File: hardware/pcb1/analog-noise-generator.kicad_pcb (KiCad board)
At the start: 4 copper layers, 12.7 x 53 mm, 79 parts, among them J1 USB_C_Receptacle_USB2.0, J2 Conn_01x03_Pin, J5 Conn_01x04_Pin, J6 Conn_01x04_Pin, J7 Conn_01x02_Pin, J9 Conn_02x04_Odd_Even, U1 STM32F072CBTx, U2 USBLC6-2SC6, U3 LR8321A-T33, U4 LIS2DH12, U5 LM324

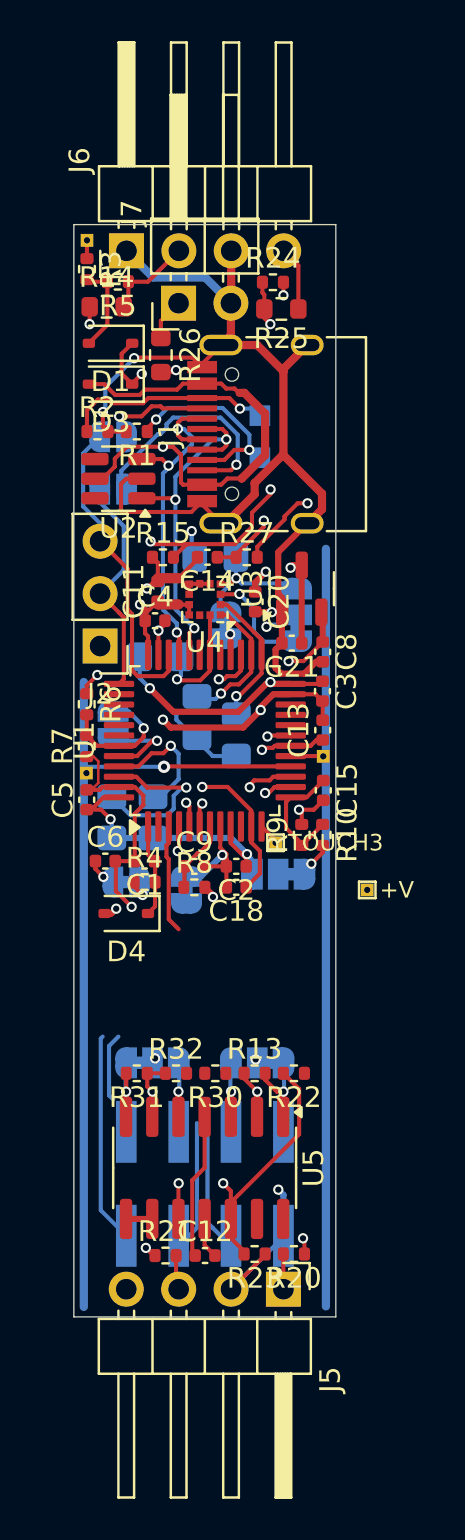
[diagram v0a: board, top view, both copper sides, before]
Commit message: finish routing
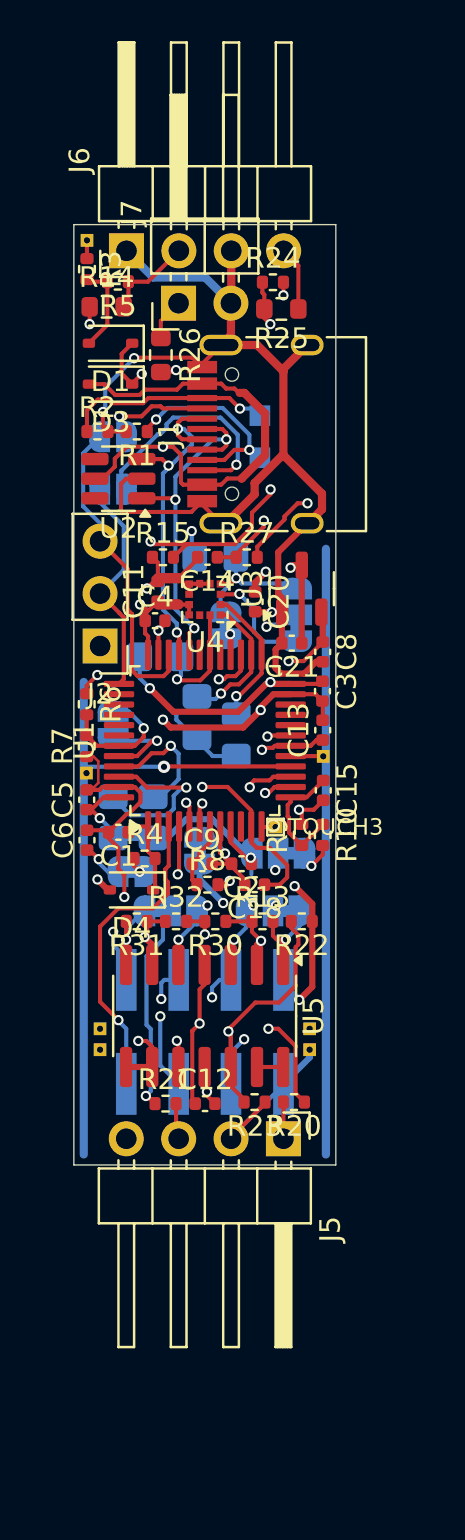
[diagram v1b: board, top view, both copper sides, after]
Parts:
- added TP10: AGND, analog-noise-generator:TestPoint_THTPad_small, B.Cu at (106.7, 96.5)
- added TP11: AVCC, analog-noise-generator:TestPoint_THTPad_small, B.Cu at (106.7, 95.5)
- added TP9: GND, analog-noise-generator:TestPoint_THTPad_small, B.Cu at (116.8, 96.5)
- TP4: moved to B.Cu
- moved JP6 7.42 mm to (110.1, 89.8)
- moved JP4 7.41 mm to (115.1, 89.8)
- moved R13 7.38 mm to (114.6, 90.3)
- moved R22 7.38 mm to (116.5, 90.3)
- moved C12 7.37 mm to (111.8, 99.1)
- moved J9 7.37 mm to (111.8, 95.7)
- moved R20 7.37 mm to (116.1, 99.1)
- moved R21 7.37 mm to (109.9, 99.1)
- moved R23 7.37 mm to (114.2, 99.1)
- moved R30 7.37 mm to (112.3, 90.3)
- moved R31 7.37 mm to (108.5, 90.3)
- moved R32 7.37 mm to (110.4, 90.3)
- moved U5 7.37 mm to (111.8, 94.9)
- moved J5 7.29 mm to (115.6, 100.8)
- moved TP4 7.29 mm to (116.8, 95.5), turned to 180 degrees
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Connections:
- U1 pad 4: /EPD_DC -> /EPD_CS
- U1 pad 5: /EPD_CS -> /EPD_RES
- U1 pad 6: /EPD_RES -> /EPD_DC
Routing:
- net /Vmiddle: track 37.7 -> 55.7 mm, vias 2 -> 3
- net /AGND: track 1.98 -> 19.4 mm, vias 0 -> 2
- net /AVCC: track 7.03 -> 22.7 mm, vias 0 -> 2
- net GND: track 148.4 -> 161.5 mm
- net +3.3V: track 69.2 -> 78.4 mm, vias 9 -> 11
- net /TOUCH1: track 40.4 -> 33.0 mm
- net /TOUCH2: track 38.5 -> 31.1 mm
- net +8V: track 43.9 -> 51.3 mm
- net /EPD_DC: track 10.3 -> 16.5 mm, vias 1 -> 2
- net /MOSI: track 16.4 -> 21.9 mm, vias 1 -> 2
- net /DAC2: track 9.72 -> 14.0 mm, vias 2 -> 3
- net /EPD_CS: track 6.73 -> 10.4 mm, vias 1 -> 2
- net /SCK: track 24.1 -> 27.8 mm, vias 1 -> 2
- net /DAC1: track 8.41 -> 11.6 mm, vias 2 -> 3
- net /EPD_RES: track 10.1 -> 11.5 mm, vias 1 -> 2
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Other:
- board size 12.7 x 53 mm -> 12.7 x 45.6 mm

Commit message: improve silk
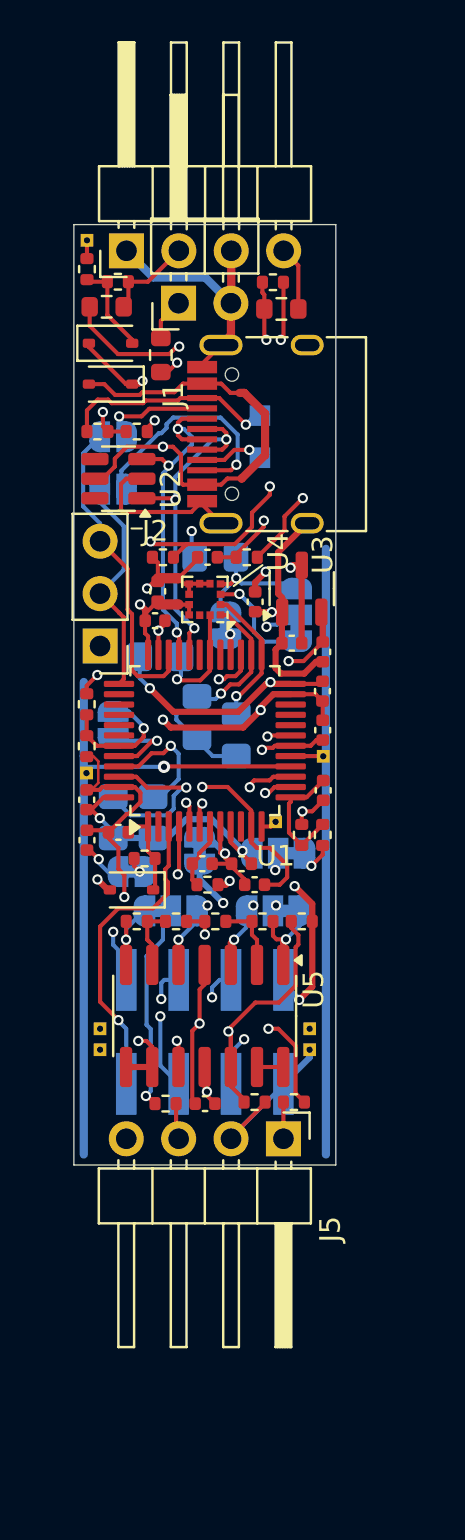
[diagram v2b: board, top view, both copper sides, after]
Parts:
- added QR1: QR_git_3.8, analog-noise-generator-qr:QR_git_3.8, B.Cu at (107.6, 61.8)
- TP6: value TOUCH1 -> T1
- TP7: value TOUCH2 -> T2
- TP8: value TOUCH3 -> T3; moved to B.Cu
- moved TP8 0.25 mm to (115.2, 85.5), turned to 180 degrees
- turned D1 to 0 degrees
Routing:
- net /IN2L: track 32.4 -> 28.9 mm
- net +8V: track 51.3 -> 49.8 mm
- net GND: track 161.5 -> 160.7 mm, vias 11 -> 10
- net Net-(J1-CC1): track 9.95 -> 9.31 mm
- net /Vmiddle: track 55.7 -> 55.1 mm
- net /VIN_sense: track 47.0 -> 47.5 mm
- net +3.3V: track 78.4 -> 77.9 mm
- net Net-(U5A--): track 3.64 -> 3.48 mm, vias 1 -> 0
- net Net-(U5B--): track 3.20 -> 3.10 mm, vias 1 -> 0
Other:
- board text added: "1"
- board text added: "2"
- board text added: "3V3"
- board text added: "G"
- board text added: "GATE"
- board text added: "GND"
- board text added: "IN1"
- board text added: "IN2"
- board text added: "SWCLK"
- board text added: "SWDIO"
- board text added: "analog noise"
- board text added: "snowball"
- board text added: "v1"
